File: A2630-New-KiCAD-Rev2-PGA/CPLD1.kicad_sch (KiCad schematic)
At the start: 19 parts, among them CN600 CPLD0, CN601 CPLD1, CN602 CPLD2, J600 IDE DISABLE, U600 XC9572XL-VQ64, U601 XC95144XL-TQ144, U602 XC95144XL-TQ144

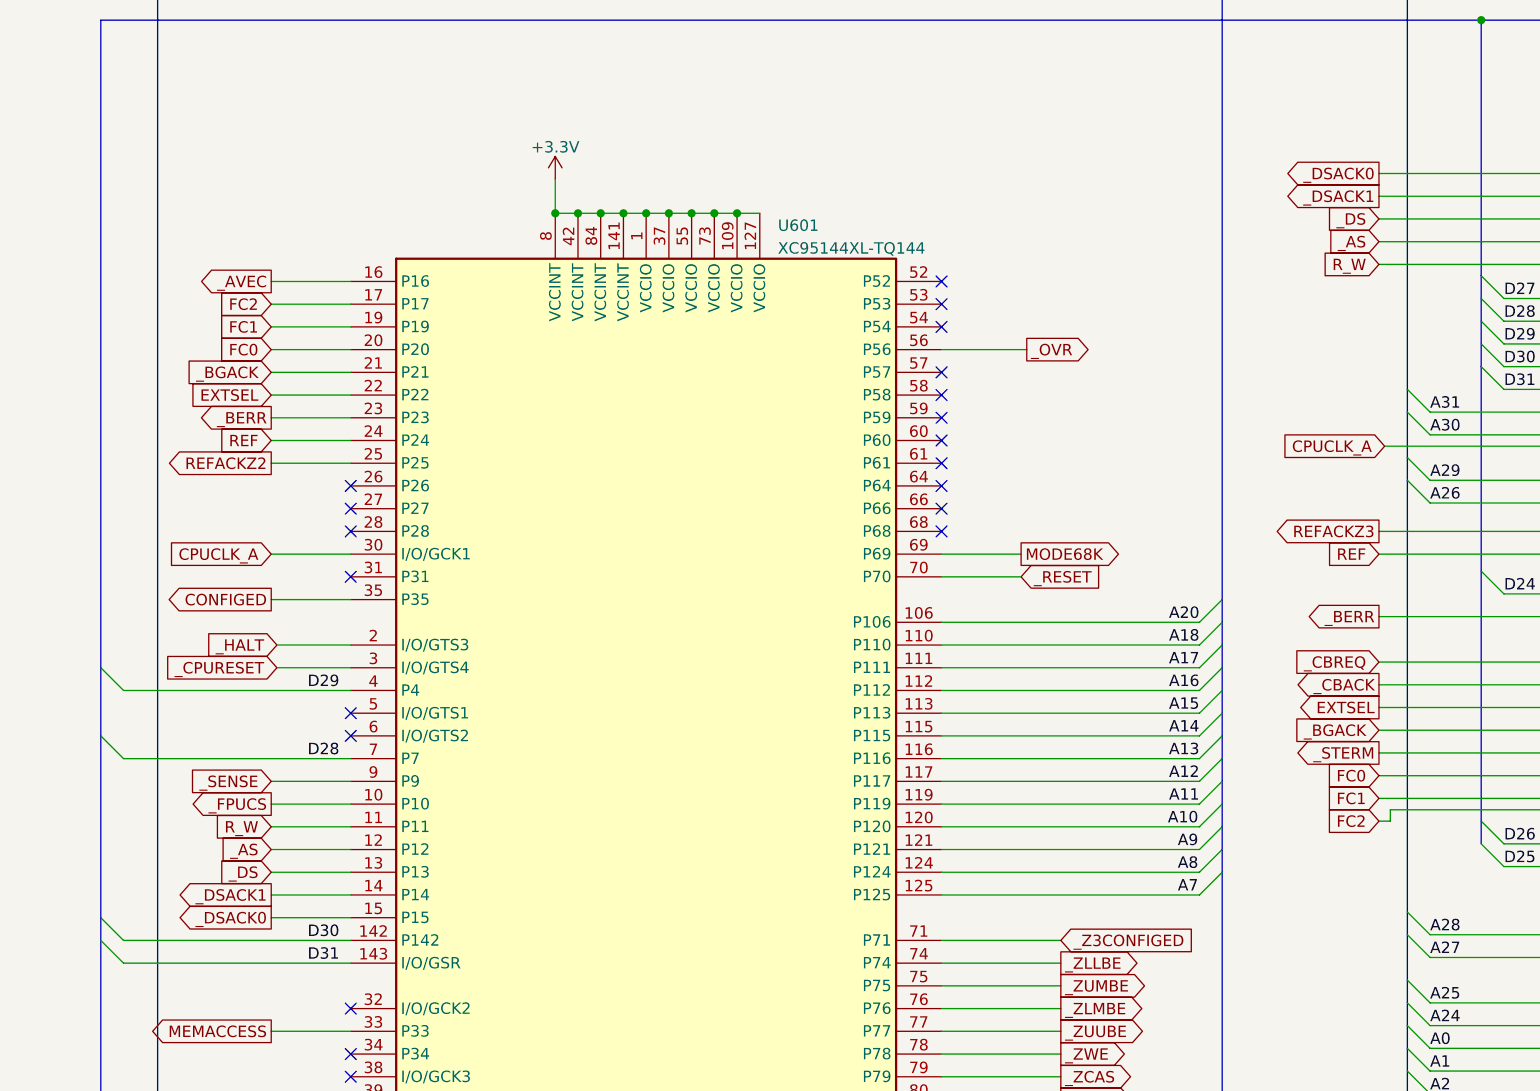
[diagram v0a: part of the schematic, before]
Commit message: Add files via upload
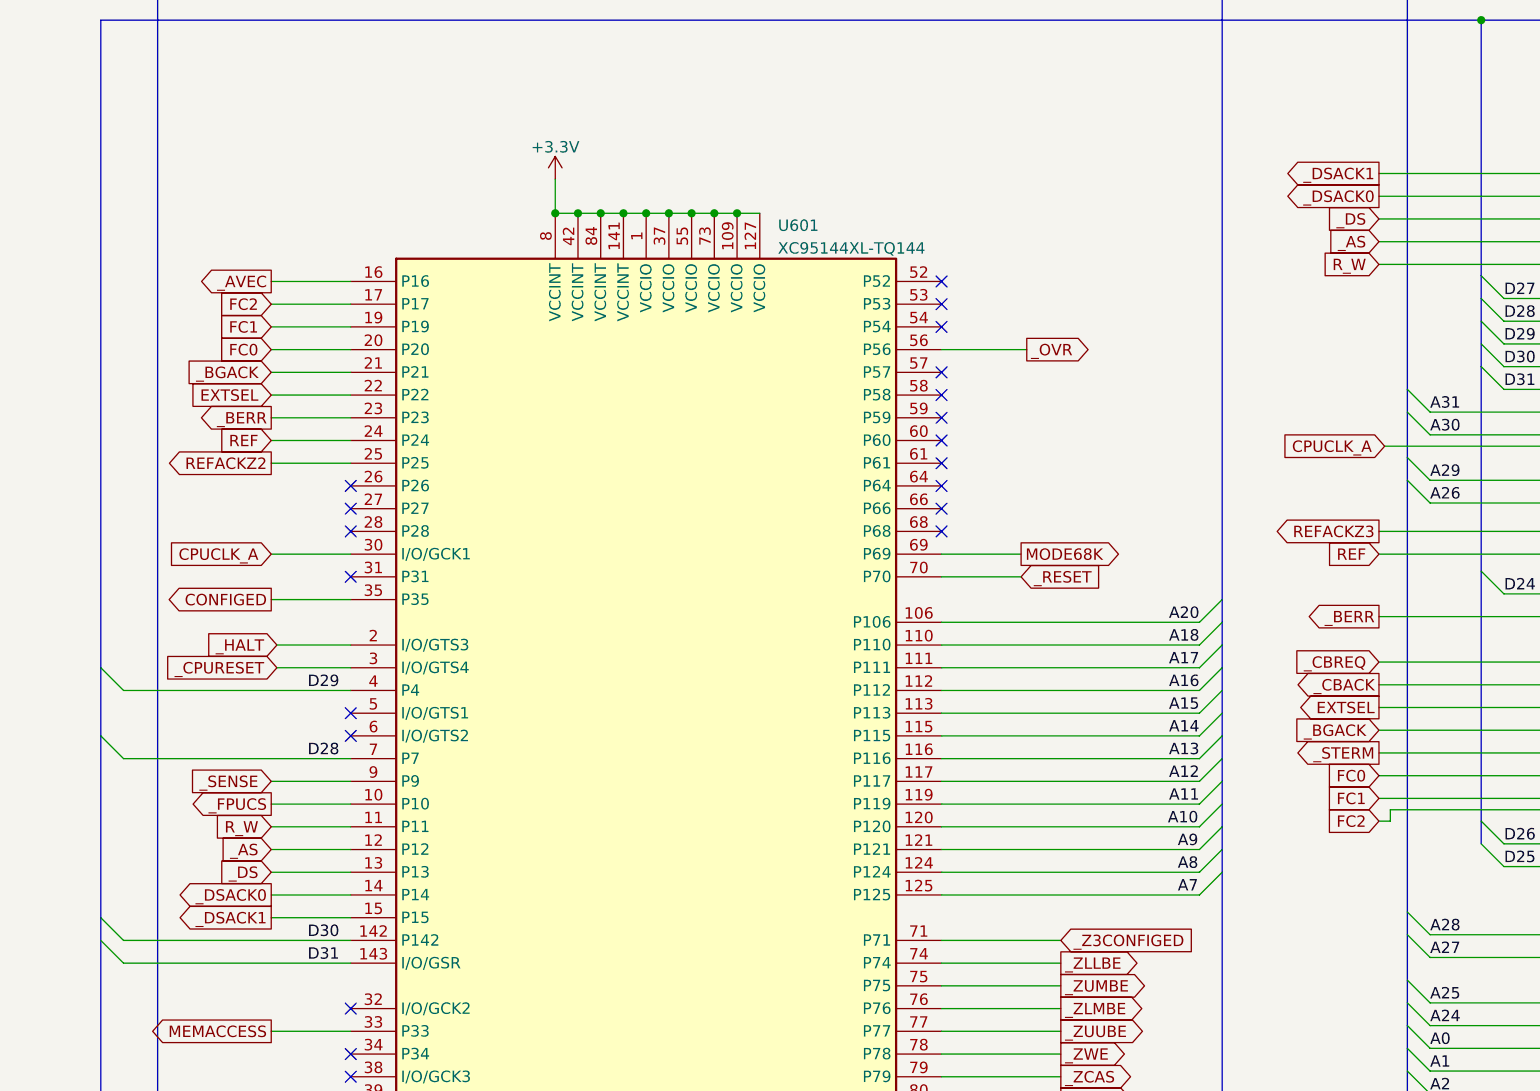
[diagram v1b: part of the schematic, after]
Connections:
- net _DSACK0: now also U601.14 (P14), U602.17 (P17); no longer U601.15 (P15), U602.16 (P16)
- net _DSACK1: now also U601.15 (P15), U602.16 (P16); no longer U601.14 (P14), U602.17 (P17)
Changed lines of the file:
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@@
     )
   )
-  (global_label "_DSACK1" (shape output) (at 151.765 133.35 180) (fields_autoplaced)
-    (effects (font (size 1.27 1.27)) (justify right))
-    (property "Intersheet References" "${INTERSHEET_REFS}" (id 0) (at 262.255 240.665 0)
-      (effects (font (size 1.27 1.27)) hide)
+  (global_label "_DSACK0" (shape output) (at 151.765 133.35 180) (fields_autoplaced)
+    (effects (font (size 1.27 1.27)) (justify right))
+    (property "Intersheet References" "${INTERSHEET_REFS}" (id 0) (at 141.1556 133.2706 0)
+      (effects (font (size 1.27 1.27)) (justify right) hide)
     )
   )
@@
     )
   )
-  (global_label "_DSACK0" (shape output) (at 275.59 52.705 180) (fields_autoplaced)
-    (effects (font (size 1.27 1.27)) (justify right))
-    (property "Intersheet References" "${INTERSHEET_REFS}" (id 0) (at 386.08 162.56 0)
-      (effects (font (size 1.27 1.27)) hide)
+  (global_label "_DSACK1" (shape output) (at 275.59 52.705 180) (fields_autoplaced)
+    (effects (font (size 1.27 1.27)) (justify right))
+    (property "Intersheet References" "${INTERSHEET_REFS}" (id 0) (at 264.9806 52.6256 0)
+      (effects (font (size 1.27 1.27)) (justify right) hide)
     )
   )
@@
     )
   )
-  (global_label "_DSACK1" (shape output) (at 275.59 55.245 180) (fields_autoplaced)
-    (effects (font (size 1.27 1.27)) (justify right))
-    (property "Intersheet References" "${INTERSHEET_REFS}" (id 0) (at 386.08 162.56 0)
-      (effects (font (size 1.27 1.27)) hide)
-    )
-  )
-  (global_label "_DSACK0" (shape output) (at 151.765 135.89 180) (fields_autoplaced)
-    (effects (font (size 1.27 1.27)) (justify right))
-    (property "Intersheet References" "${INTERSHEET_REFS}" (id 0) (at 262.255 245.745 0)
-      (effects (font (size 1.27 1.27)) hide)
-    )
-  )
+  (global_label "_DSACK0" (shape output) (at 275.59 55.245 180) (fields_autoplaced)
+    (effects (font (size 1.27 1.27)) (justify right))
+    (property "Intersheet References" "${INTERSHEET_REFS}" (id 0) (at 264.9806 55.1656 0)
+      (effects (font (size 1.27 1.27)) (justify right) hide)
+    )
+  )
+  (global_label "_DSACK1" (shape output) (at 151.765 135.89 180) (fields_autoplaced)
+    (effects (font (size 1.27 1.27)) (justify right))
+    (property "Intersheet References" "${INTERSHEET_REFS}" (id 0) (at 141.1556 135.8106 0)
+      (effects (font (size 1.27 1.27)) (justify right) hide)
+    )
+  )
